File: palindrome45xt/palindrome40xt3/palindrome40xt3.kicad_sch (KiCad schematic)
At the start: 110 parts, among them J1 Conn_01x02_Socket, Q1 Q_NMOS_GDS, Q3 TIP120, U1 RP2040_Zero

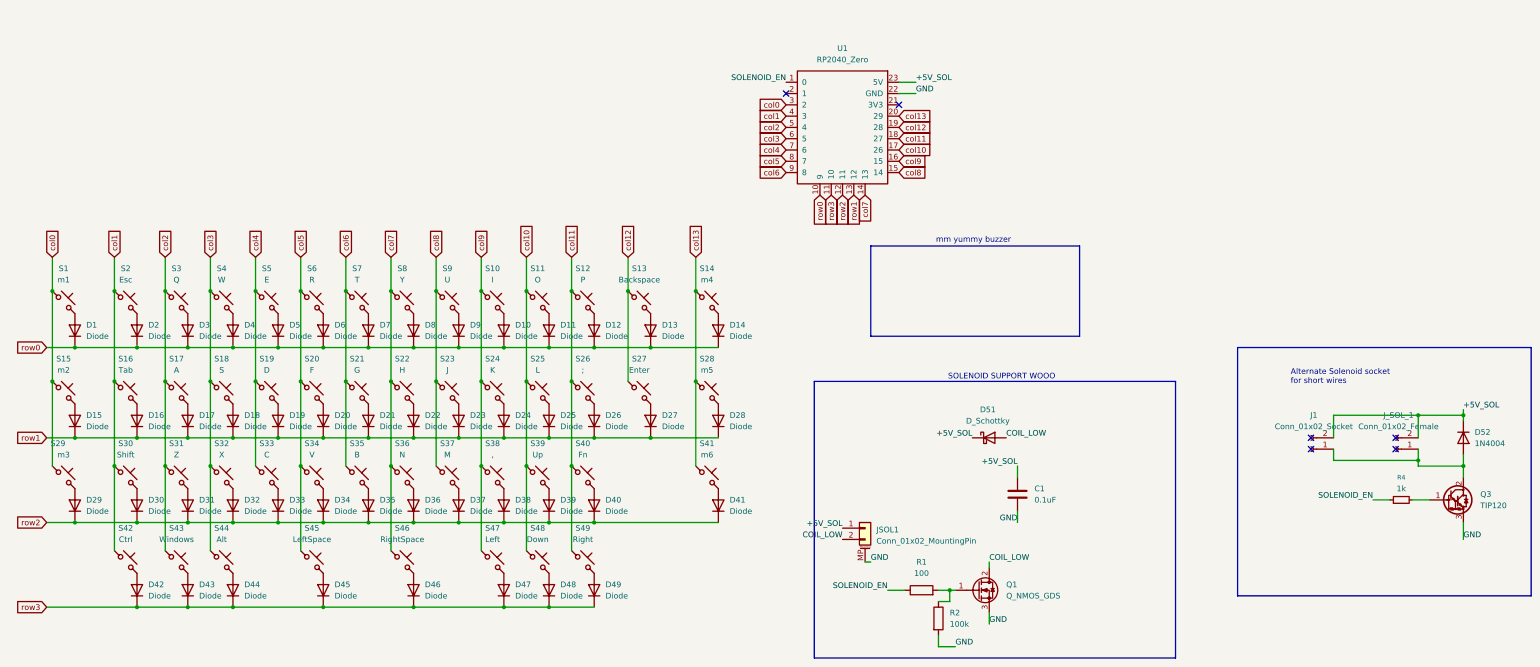
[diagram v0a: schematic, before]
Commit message: disaster here
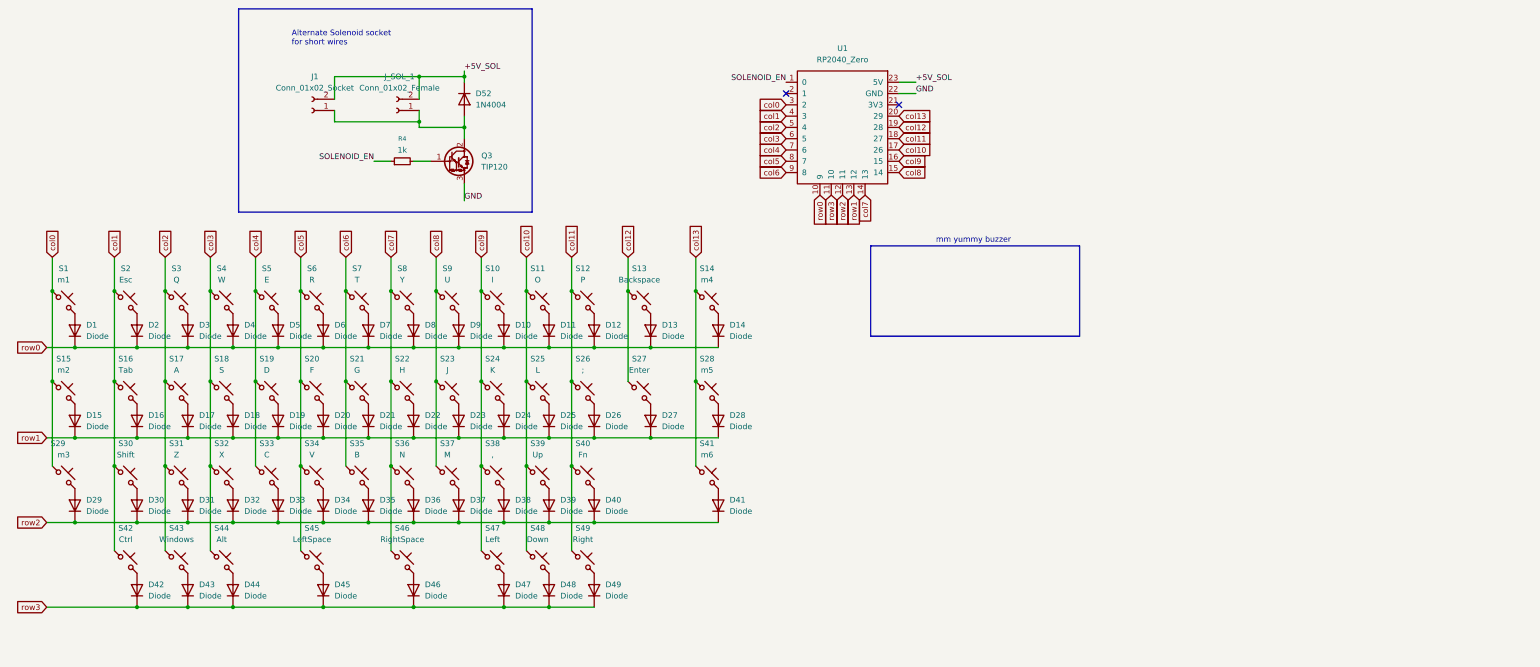
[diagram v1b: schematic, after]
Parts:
- removed C1: 0.1uF, Capacitor_SMD:C_0805_2012Metric, symbol Device:C
- removed D51: D_Schottky, Diode_SMD:D_SOD-123, symbol Device:D_Schottky
- removed JSOL1: Conn_01x02_MountingPin, Connector_JST:JST_SH_SM02B-SRSS-TB_1x02-1MP_P1.00mm_Horizontal, symbol Connector_Generic_MountingPin:Conn_01x02_MountingPin
- removed Q1: Q_NMOS_GDS, Package_TO_SOT_THT:TO-220-3_Horizontal_TabDown, symbol Transistor_FET:Q_NMOS_GDS
- removed R1: 100, Resistor_SMD:R_0805_2012Metric, symbol Device:R
- removed R2: 100k, Resistor_SMD:R_0805_2012Metric, symbol Device:R
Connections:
- no-connect marks 6 -> 2
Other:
- note removed: "SOLENOID SUPPORT WOOO"
- moved on the sheet: D52, J1, J_SOL_1, Q3, R4
